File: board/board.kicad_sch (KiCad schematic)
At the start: 1 part

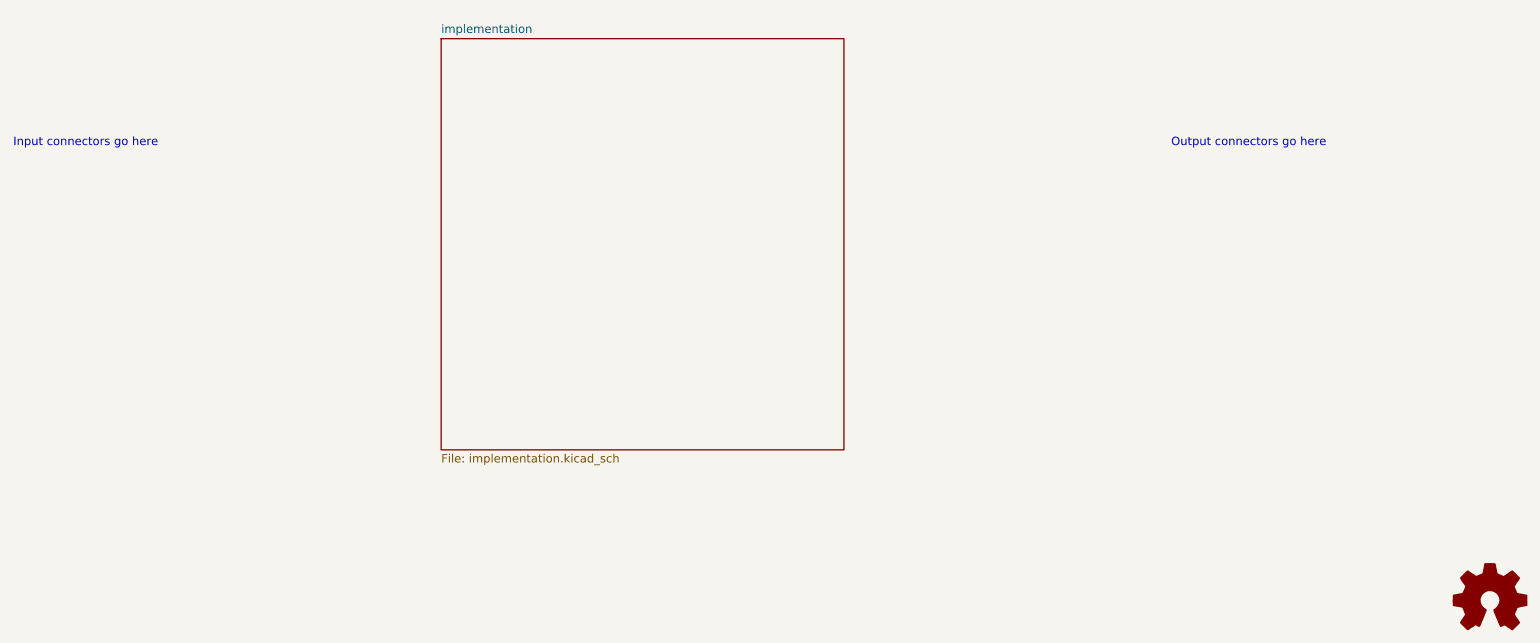
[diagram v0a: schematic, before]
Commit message: initial
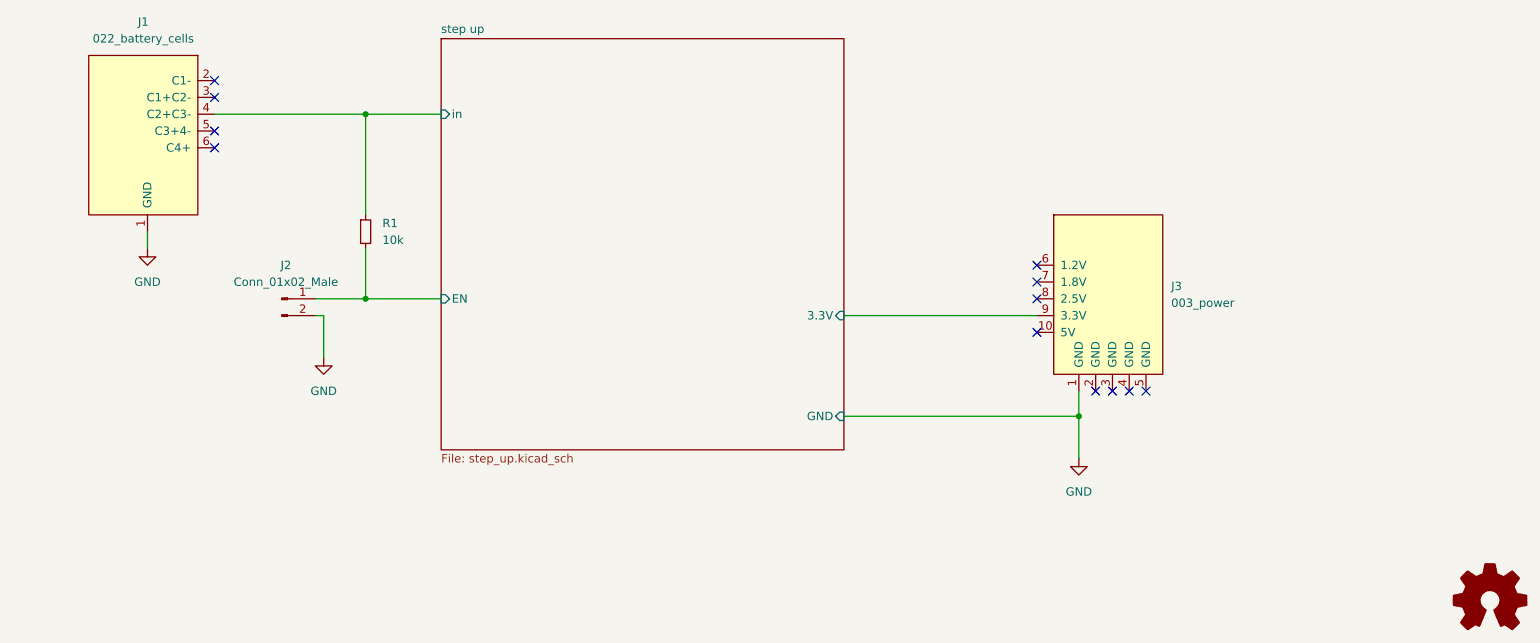
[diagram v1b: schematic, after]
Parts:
- added J1: 022_battery_cells, on_edge:on_edge_2x05_device, symbol put_on_edge:022_battery_cells
- added J2: Conn_01x02_Male, Connector_PinHeader_2.54mm:PinHeader_1x02_P2.54mm_Vertical, symbol Connector:Conn_01x02_Male
- added J3: 003_power, on_edge:on_edge_2x05_host, symbol put_on_edge:003_power
- added R1: 10k, Resistor_SMD:R_0603_1608Metric, symbol Device:R_Small
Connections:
- new net GND: J1.1 (GND), J2.2 (Pin_2), J3.1 (GND)
- new net step up/3.3V: J3.9 (3.3V)
- new net step up/EN: J2.1 (Pin_1), R1.2
- new net step up/in: J1.4 (C2+C3-), R1.1
- no-connect marks 0 -> 12
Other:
- sheet implementation renamed step up
- sheet step up: file implementation.kicad_sch -> step_up.kicad_sch
- sheet step up ports: added 3.3V, EN, GND, in; removed none
- note removed: "Input connectors go here"
- note removed: "Output connectors go here"
